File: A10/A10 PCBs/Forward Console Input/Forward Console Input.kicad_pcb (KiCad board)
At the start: 2 copper layers, 99.7 x 98.4 mm, 68 parts, among them J1 PATCH, J10 ROWS, J11 COLUMNS, J12 PATCH, J13 PATCH, J14 PWM, J15 PWM, J16 Communication, J17 PATCH, J18 PATCH, J19 PATCH, J2 FIRE HANDLES, J20 PATCH, J21 Analog, J22 Analog, J23 PATCH, J24 PATCH, J25 Power, J26 Power, J27 Analog, J28 Analog, J29 Digital, J3 UFC COLS, J30 PWM, J31 PWM, J32 Communication, J4 UFC ROWS, J5 PATCH, J6 JAMMER, J7 LANDING GEAR, J8 MASTER ARM, J9 NMSP CMSP, U1 USR-ES1

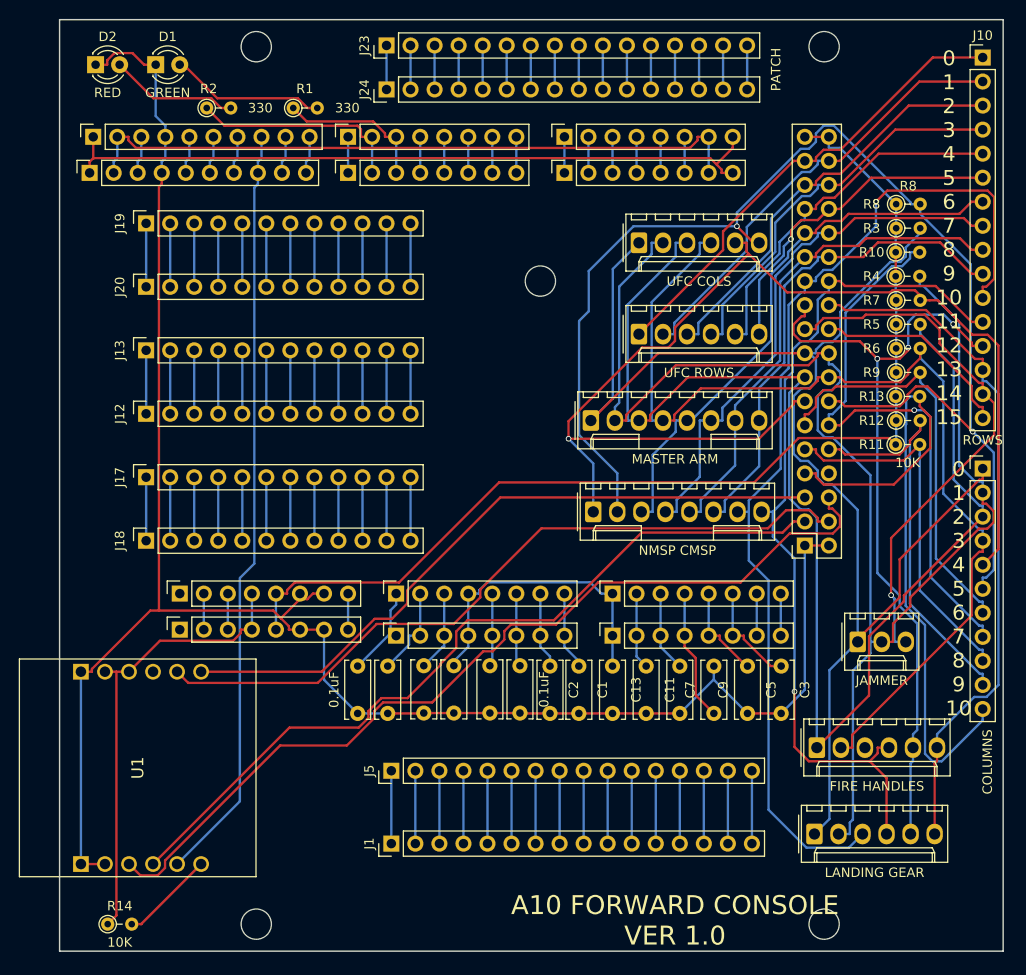
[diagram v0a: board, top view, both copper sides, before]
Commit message: A10
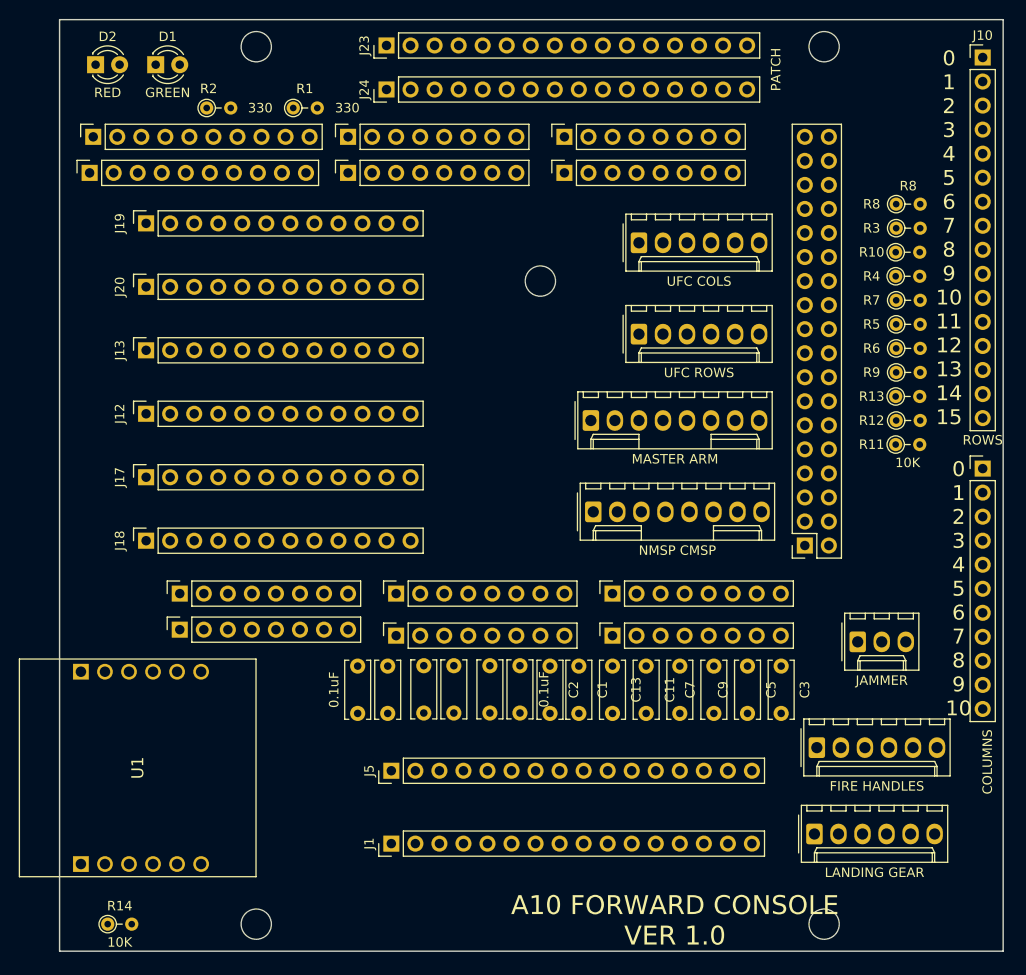
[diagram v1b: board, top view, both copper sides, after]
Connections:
- R1 pad 1: /*5 -> /*13
- R2 pad 1: /*6 -> /*12
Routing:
- net GND: track 205.5 -> 0.00 mm
- net /39: track 155.7 -> 0.00 mm
- net /38: track 148.8 -> 0.00 mm
- net /43: track 139.9 -> 0.00 mm, vias 2 -> 0
- net /40: track 139.5 -> 0.00 mm
- net /42: track 122.0 -> 0.00 mm, vias 1 -> 0
- net +5V: track 115.4 -> 0.00 mm
- net /32: track 110.1 -> 0.00 mm, vias 1 -> 0
- net /41: track 107.7 -> 0.00 mm
- net MOSI: track 96.1 -> 0.00 mm
- net /33: track 92.5 -> 0.00 mm, vias 1 -> 0
- net SCLK: track 85.4 -> 0.00 mm
- net /34: track 82.3 -> 0.00 mm, vias 3 -> 0
- net SS: track 80.5 -> 0.00 mm
- net ES1_RST: track 78.1 -> 0.00 mm
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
